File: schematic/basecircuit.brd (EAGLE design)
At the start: 65.7 x 58.4 mm, 29 parts, among them IC1 ATMEGA328-20P, Q1 16 Mhz, T1 BC337

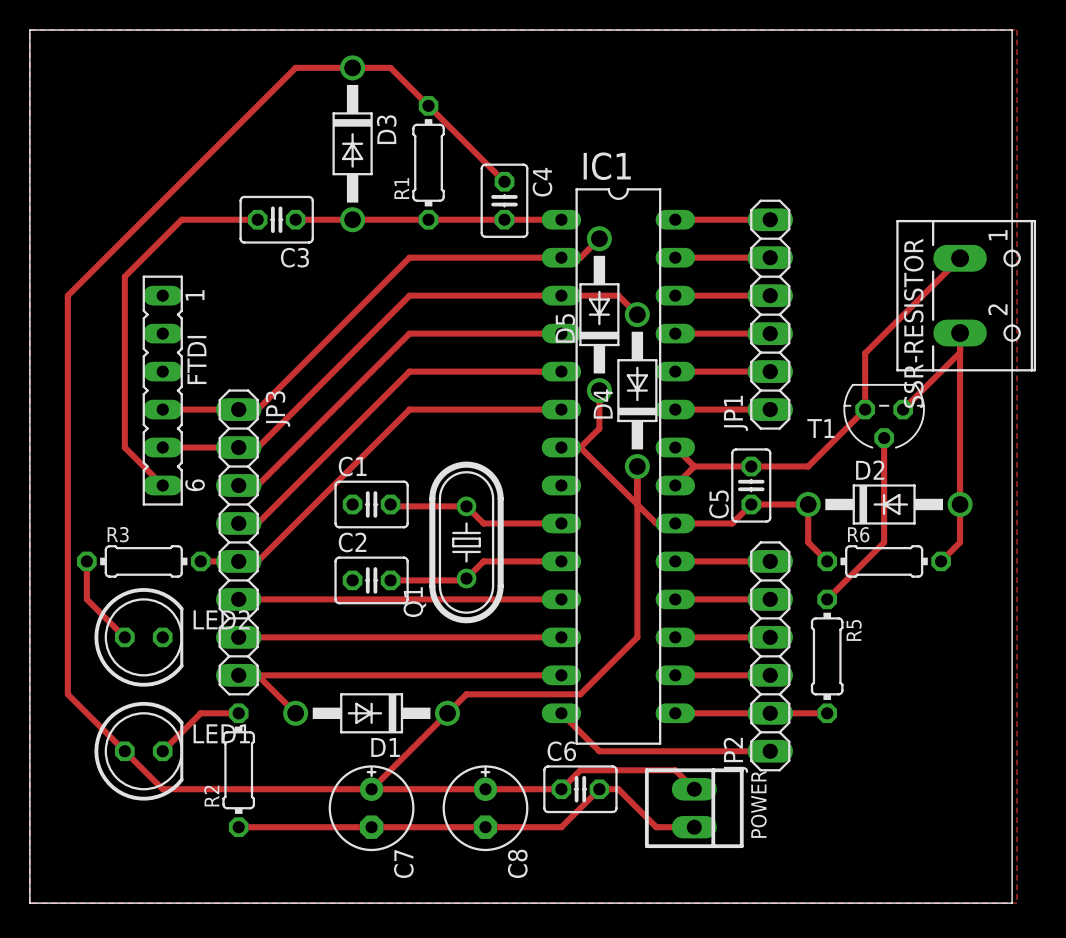
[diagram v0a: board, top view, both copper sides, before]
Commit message: some optimization
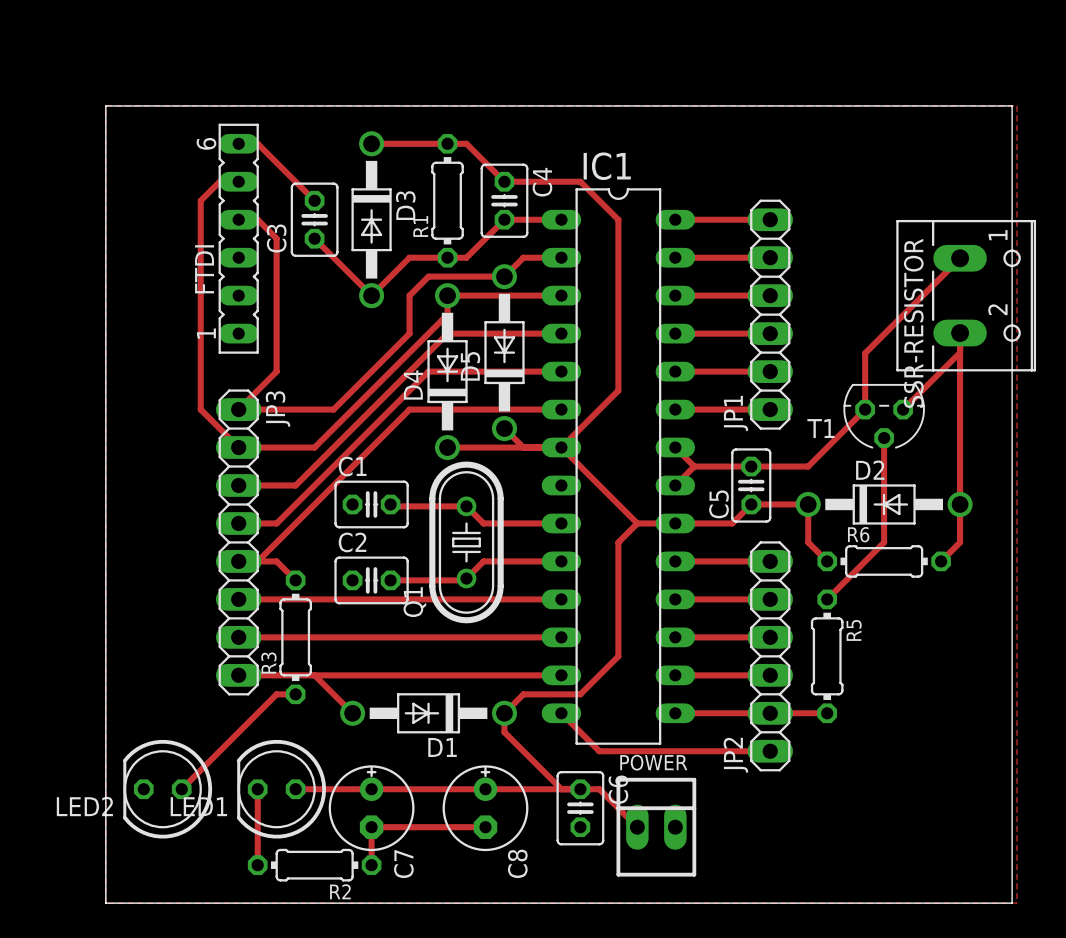
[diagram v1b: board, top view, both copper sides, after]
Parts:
- moved D4 12.8 mm to (36.8, 47.0)
- moved FTDI 11.4 mm to (22.9, 55.9), turned to 90 degrees
- moved R3 11.4 mm to (26.7, 29.2), turned to 90 degrees
- moved LED2 10.2 mm to (17.8, 19.1), turned to 180 degrees
- moved LED1 9.25 mm to (25.4, 19.1), turned to 180 degrees
- moved R2 8.13 mm to (27.9, 14.0), turned to 180 degrees
- moved D5 6.84 mm to (40.6, 48.3)
- moved D3 5.24 mm to (31.8, 57.1)
- moved D1 3.81 mm to (35.6, 24.1)
- moved POWER 2.84 mm to (50.8, 16.5), turned to 0 degrees
- moved R1 2.84 mm to (36.8, 58.4)
- moved C3 2.54 mm to (27.9, 57.1), turned to 90 degrees
- moved C6 1.27 mm to (45.7, 17.8), turned to 270 degrees
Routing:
- net VCC: track 174.7 -> 121.3 mm
- net AGND: track 61.9 -> 39.5 mm
- net N$3: track 25.5 -> 6.66 mm
- net PD1: track 36.5 -> 47.2 mm
- net PD0: track 33.9 -> 42.8 mm
- net N$6: track 6.13 -> 10.3 mm
- net N$11: track 17.8 -> 20.2 mm
- net PD4: track 28.3 -> 30.1 mm
- net N$2: track 6.13 -> 5.08 mm
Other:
- board size 65.7 x 58.4 mm -> 60.6 x 53.3 mm
